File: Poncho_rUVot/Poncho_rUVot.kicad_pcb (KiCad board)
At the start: 2 copper layers, 91.8 x 81 mm, 20 parts, among them J1 Screw_Terminal_01x03, K1 SANYOU_SRD_Form_C, P1 Conn_01x03, P2 Conn_01x03, P3 Conn_01x04, P4 Conn_01x03, P5 Conn_01x02, P6 Conn_01x02, P7 Conn_01x06, P8 Conn_01x04, P9 Conn_01x08, Q1 BC548, Q2 BC548

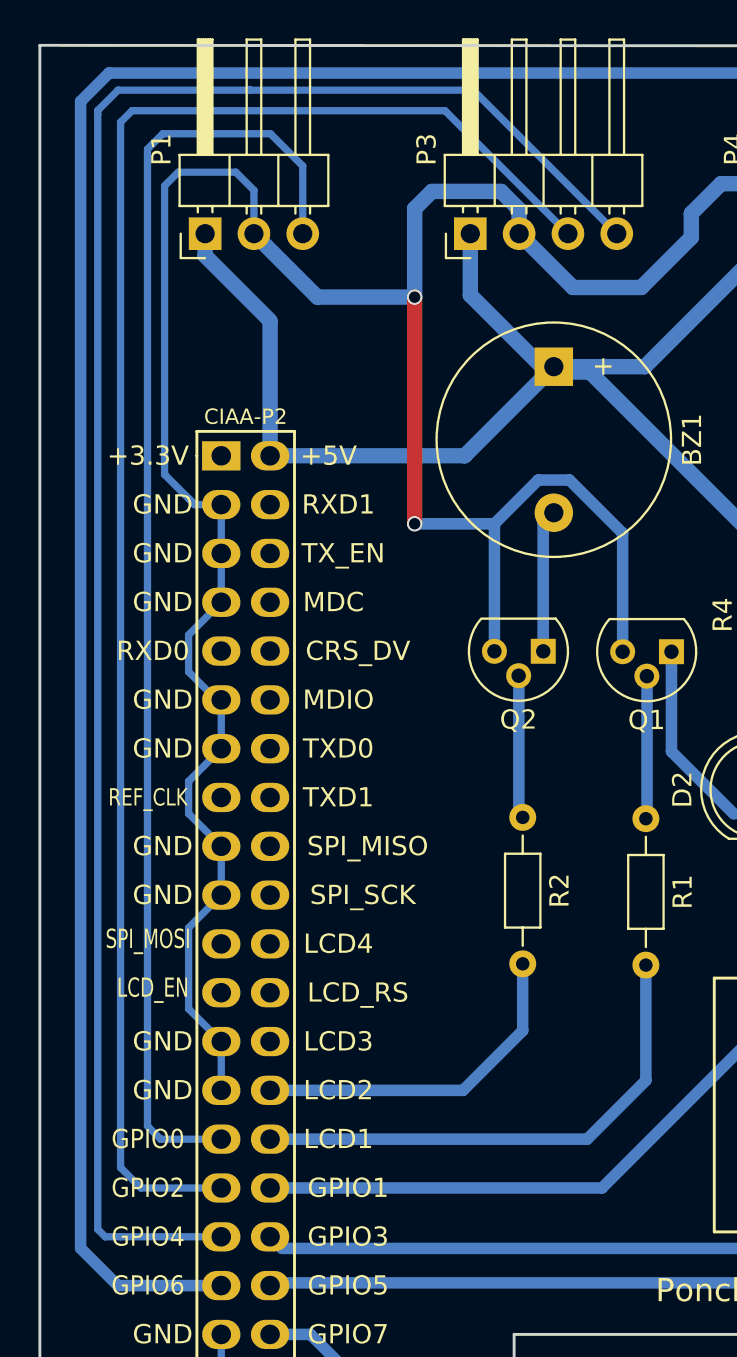
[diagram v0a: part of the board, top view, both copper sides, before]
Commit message: Correcciones
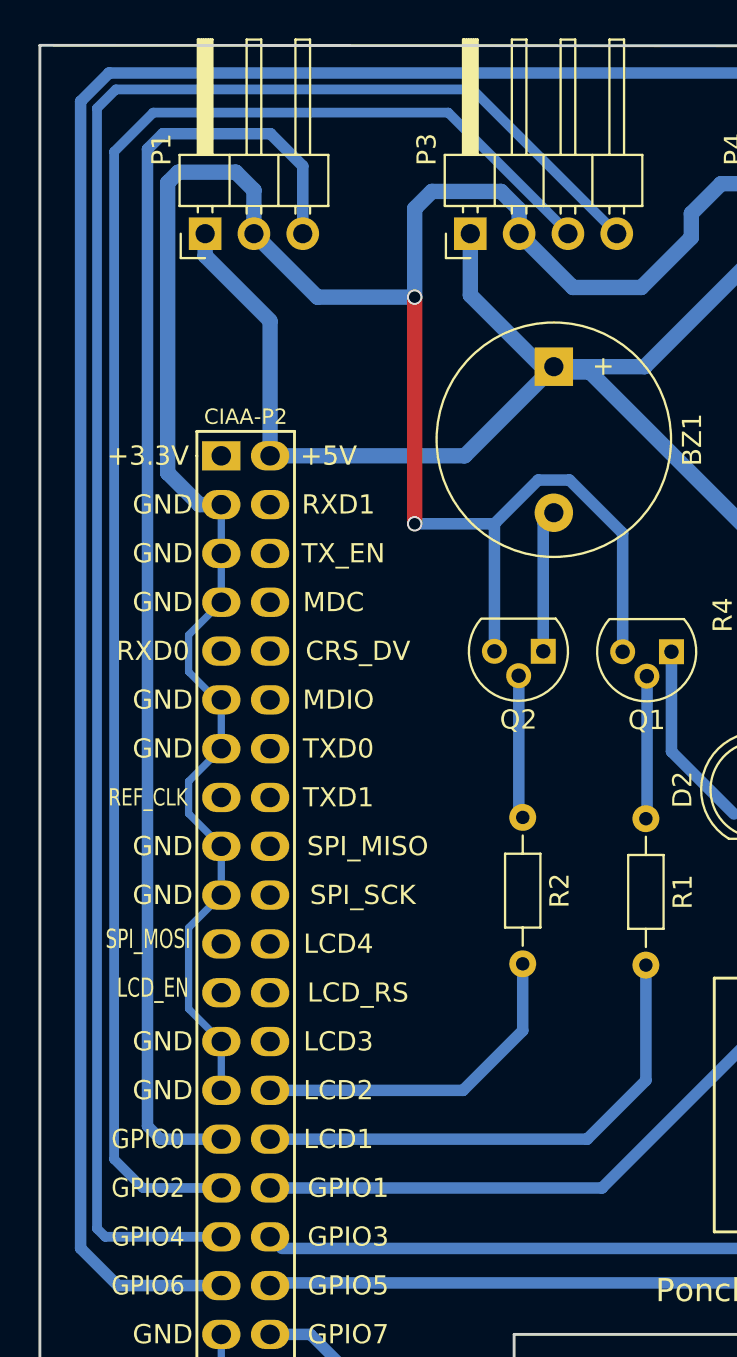
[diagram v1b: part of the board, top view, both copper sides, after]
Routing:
- net GND: track 381.1 -> 380.4 mm
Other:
- board text added: "Diseño simple faz. Sin requerimientos especiales. pistas: 0,6 mm y 0,8mm Margen: Distancia al borde: Documentaciòn superficial: HASL"
- board text removed: "Diseño simple faz. Sin requerimientos especiales."
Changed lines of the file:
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@@
     (thickness 1.6)
     (drawings 42)
-    (tracks 280)
+    (tracks 277)
     (zones 0)
     (modules 20)
@@
     (mod_text_size 0.15 0.15)
     (mod_text_width 0.02)
-    (pad_size 1.4 1.4)
-    (pad_drill 0.6)
+    (pad_size 2.6 2.6)
+    (pad_drill 1.3)
     (pad_to_mask_clearance 0.2)
     (aux_axis_origin 0 0)
@@
   (gr_line (start 148.4 146) (end 121.92 146) (angle 90) (layer Edge.Cuts) (width 0.15))
   (gr_line (start 148.4 75) (end 148.4 146) (angle 90) (layer Edge.Cuts) (width 0.15))
-  (gr_text "Diseño simple faz.\nSin requerimientos especiales." (at 194.945 24.13) (layer Dwgs.User)
-    (effects (font (size 1.5 1.5) (thickness 0.3)) (justify left))
+  (gr_text "Diseño simple faz.\nSin requerimientos especiales.\npistas: 0,6 mm y 0,8mm \nMargen: \nDistancia al borde: \nDocumentaciòn superficial: HASL\n" (at 191.75 33.25) (layer Dwgs.User)
+    (effects (font (size 1.8 1.8) (thickness 0.4)) (justify left))
   )
   (gr_text STACK-UP (at 227.965 19.05) (layer Dwgs.User)
-    (effects (font (size 1.5 1.5) (thickness 0.3)))
+    (effects (font (size 1.8 1.8) (thickness 0.4)))
   )
   (gr_line (start 278.765 16.51) (end 186.69 16.51) (angle 90) (layer Dwgs.User) (width 0.2))
@@
   (segment (start 66.04 109.22) (end 64.33949 110.92051) (width 0.381) (layer B.Cu) (net 2))
   (segment (start 66.04 116.84) (end 66.04 119.38) (width 0.381) (layer B.Cu) (net 2))
-  (segment (start 67.74 72.54) (end 67.74 74.8) (width 0.381) (layer B.Cu) (net 2))
-  (segment (start 64.659 88.9) (end 63.09101 87.33201) (width 0.381) (layer B.Cu) (net 2))
-  (segment (start 63.09101 87.33201) (end 63.09101 72.30899) (width 0.381) (layer B.Cu) (net 2))
-  (segment (start 66.04 88.9) (end 64.659 88.9) (width 0.381) (layer B.Cu) (net 2))
-  (segment (start 63.09101 72.30899) (end 63.8 71.6) (width 0.381) (layer B.Cu) (net 2))
-  (segment (start 63.8 71.6) (end 66.8 71.6) (width 0.381) (layer B.Cu) (net 2))
-  (segment (start 66.8 71.6) (end 67.74 72.54) (width 0.381) (layer B.Cu) (net 2))
-  (segment (start 64.659 88.9) (end 64.339499 88.580499) (width 0.381) (layer B.Cu) (net 2))
+  (segment (start 67.74 72.54) (end 67.74 74.8) (width 0.8) (layer B.Cu) (net 2))
+  (segment (start 63.8 71.6) (end 66.8 71.6) (width 0.8) (layer B.Cu) (net 2))
+  (segment (start 66.8 71.6) (end 67.74 72.54) (width 0.8) (layer B.Cu) (net 2))
   (segment (start 86.92684 90.387038) (end 86.92684 90.67316) (width 0.381) (layer B.Cu) (net 2))
   (segment (start 80.25384 89.896398) (end 80.25384 96.5327) (width 0.6) (layer B.Cu) (net 2))
@@
   (segment (start 92.05 72.2) (end 95.2 72.2) (width 0.8) (layer B.Cu) (net 2))
   (segment (start 90.5 73.75) (end 92.05 72.2) (width 0.8) (layer B.Cu) (net 2))
+  (segment (start 66.04 88.9) (end 64.9 88.9) (width 0.8) (layer B.Cu) (net 2))
+  (segment (start 64.9 88.9) (end 63.25 87.25) (width 0.8) (layer B.Cu) (net 2))
+  (segment (start 63.25 72.15) (end 63.8 71.6) (width 0.8) (layer B.Cu) (net 2))
+  (segment (start 63.25 87.25) (end 63.25 72.15) (width 0.8) (layer B.Cu) (net 2))
   (segment (start 136.922 109.22) (end 137.16 109.22) (width 1) (layer F.Cu) (net 9))
   (segment (start 137.16 109.22) (end 134.03 109.22) (width 0.6) (layer B.Cu) (net 9))
@@
   (segment (start 78.62 119.38) (end 68.58 119.38) (width 0.6) (layer B.Cu) (net 41))
   (segment (start 81.72704 116.27296) (end 78.62 119.38) (width 0.6) (layer B.Cu) (net 41))
-  (segment (start 66.04 121.92) (end 62.88 121.92) (width 0.381) (layer B.Cu) (net 42))
-  (segment (start 62.88 121.92) (end 62.2 121.24) (width 0.381) (layer B.Cu) (net 42))
-  (segment (start 62.2 121.24) (end 62.2 70.4) (width 0.381) (layer B.Cu) (net 42))
-  (segment (start 62.2 70.4) (end 63 69.6) (width 0.381) (layer B.Cu) (net 42))
-  (segment (start 63 69.6) (end 68.6 69.6) (width 0.381) (layer B.Cu) (net 42))
-  (segment (start 70.28 71.28) (end 70.28 74.8) (width 0.381) (layer B.Cu) (net 42))
-  (segment (start 68.6 69.6) (end 70.28 71.28) (width 0.381) (layer B.Cu) (net 42))
+  (segment (start 66.04 121.92) (end 62.88 121.92) (width 0.6) (layer B.Cu) (net 42))
+  (segment (start 62.88 121.92) (end 62.2 121.24) (width 0.6) (layer B.Cu) (net 42))
+  (segment (start 62.2 121.24) (end 62.2 70.4) (width 0.6) (layer B.Cu) (net 42))
+  (segment (start 62.2 70.4) (end 63 69.6) (width 0.6) (layer B.Cu) (net 42))
+  (segment (start 63 69.6) (end 68.6 69.6) (width 0.6) (layer B.Cu) (net 42))
+  (segment (start 70.28 71.28) (end 70.28 74.8) (width 0.6) (layer B.Cu) (net 42))
+  (segment (start 68.6 69.6) (end 70.28 71.28) (width 0.6) (layer B.Cu) (net 42))
   (segment (start 88.13546 112.86236) (end 88.13546 118.86454) (width 0.6) (layer B.Cu) (net 43))
   (segment (start 85.08 121.92) (end 68.58 121.92) (width 0.6) (layer B.Cu) (net 43))
   (segment (start 88.13546 118.86454) (end 85.08 121.92) (width 0.6) (layer B.Cu) (net 43))
-  (segment (start 66.04 124.46) (end 61.86 124.46) (width 0.381) (layer B.Cu) (net 44))
-  (segment (start 61.86 124.46) (end 60.8 123.4) (width 0.381) (layer B.Cu) (net 44))
-  (segment (start 60.8 69) (end 61.4 68.4) (width 0.381) (layer B.Cu) (net 44))
-  (segment (start 60.8 123.4) (end 60.8 69) (width 0.381) (layer B.Cu) (net 44))
-  (segment (start 77.68 68.4) (end 84.08 74.8) (width 0.381) (layer B.Cu) (net 44))
-  (segment (start 61.4 68.4) (end 77.68 68.4) (width 0.381) (layer B.Cu) (net 44))
+  (segment (start 84.08 74.57198) (end 84.08 74.8) (width 0.508) (layer B.Cu) (net 44))
+  (segment (start 66.04 124.46) (end 61.96 124.46) (width 0.508) (layer B.Cu) (net 44))
+  (segment (start 60.46502 122.96502) (end 60.46502 70.53498) (width 0.508) (layer B.Cu) (net 44))
+  (segment (start 61.96 124.46) (end 60.46502 122.96502) (width 0.508) (layer B.Cu) (net 44))
+  (segment (start 60.46502 70.53498) (end 62.5 68.5) (width 0.508) (layer B.Cu) (net 44))
+  (segment (start 84.08 74.730828) (end 84.08 74.8) (width 0.508) (layer B.Cu) (net 44))
+  (segment (start 77.849172 68.5) (end 84.08 74.730828) (width 0.508) (layer B.Cu) (net 44))
+  (segment (start 62.5 68.5) (end 77.849172 68.5) (width 0.508) (layer B.Cu) (net 44))
   (segment (start 131.08 75.92) (end 131.08 74.8) (width 0.381) (layer B.Cu) (net 45))
   (segment (start 131.08 77.92) (end 131.08 74.8) (width 0.6) (layer B.Cu) (net 45))
@@
   (segment (start 122 109) (end 122 87) (width 0.6) (layer B.Cu) (net 45))
   (segment (start 122 87) (end 131.08 77.92) (width 0.6) (layer B.Cu) (net 45))
-  (segment (start 66.04 127) (end 60.8 127) (width 0.381) (layer B.Cu) (net 46))
-  (segment (start 60 127) (end 59.61101 126.61101) (width 0.381) (layer B.Cu) (net 46))
-  (segment (start 60.8 127) (end 60 127) (width 0.381) (layer B.Cu) (net 46))
-  (segment (start 59.61101 126.61101) (end 59.61101 68.6) (width 0.381) (layer B.Cu) (net 46))
-  (segment (start 59.61101 68.38899) (end 60.66899 67.33101) (width 0.381) (layer B.Cu) (net 46))
-  (segment (start 59.61101 68.6) (end 59.61101 68.38899) (width 0.381) (layer B.Cu) (net 46))
-  (segment (start 67.46899 67.33101) (end 67.50899 67.29101) (width 0.381) (layer B.Cu) (net 46))
-  (segment (start 60.66899 67.33101) (end 67.46899 67.33101) (width 0.381) (layer B.Cu) (net 46))
-  (segment (start 79.15101 67.33101) (end 86.62 74.8) (width 0.381) (layer B.Cu) (net 46))
-  (segment (start 67.46899 67.33101) (end 79.15101 67.33101) (width 0.381) (layer B.Cu) (net 46))
+  (segment (start 79.11401 67.29401) (end 86.62 74.8) (width 0.508) (layer B.Cu) (net 46))
+  (segment (start 60.553742 67.29401) (end 79.11401 67.29401) (width 0.508) (layer B.Cu) (net 46))
+  (segment (start 59.57401 126.57401) (end 59.57401 68.273742) (width 0.508) (layer B.Cu) (net 46))
+  (segment (start 59.57401 68.273742) (end 60.553742 67.29401) (width 0.508) (layer B.Cu) (net 46))
+  (segment (start 66.04 127) (end 60 127) (width 0.508) (layer B.Cu) (net 46))
+  (segment (start 60 127) (end 59.57401 126.57401) (width 0.508) (layer B.Cu) (net 46))
   (segment (start 69.185791 127.605791) (end 68.58 127) (width 0.381) (layer B.Cu) (net 47))
   (segment (start 125.2 129.2) (end 123.605791 127.605791) (width 0.6) (layer B.Cu) (net 47))
